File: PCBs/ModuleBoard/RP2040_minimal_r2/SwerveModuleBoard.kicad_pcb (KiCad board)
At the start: 2 copper layers, 60 x 52.9 mm, 57 parts, among them IC1 AS5600-ASOT, J1 USB_B_Micro, J2 Conn_02x02_Counter_Clockwise, J3 Conn_02x08_Odd_Even_MountingP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, J4 Conn_01x07, J5 Conn_01x06_Pin, J6 Conn_01x02, J7 Conn_01x06_Pin, U2 W25Q128JVS, U3 RP2040, U4 DRV8245HQRXZRQ1, U5 DRV8245HQRXZRQ1, U6 MIC5219-3.3YM5, Y1 ABM8-272-T3

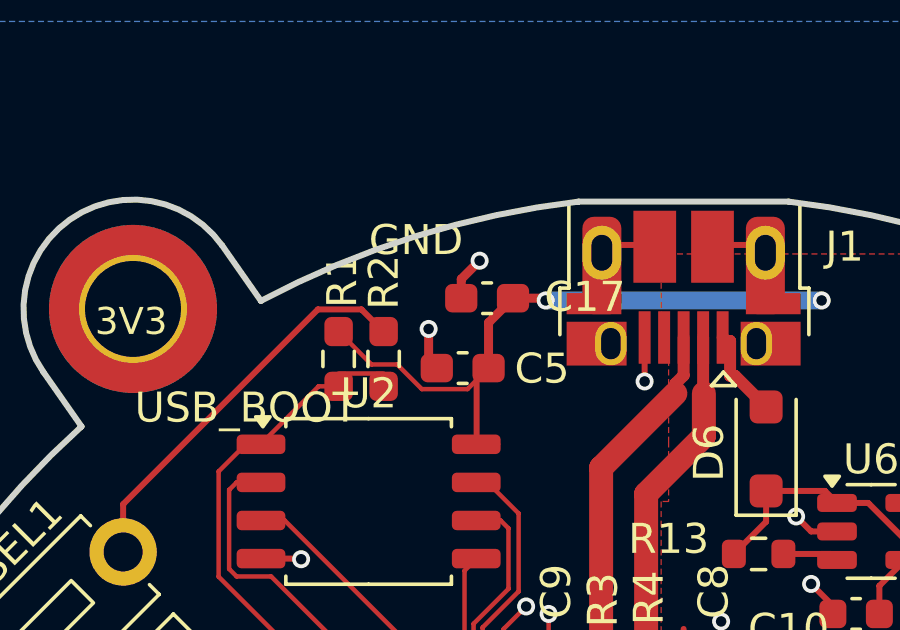
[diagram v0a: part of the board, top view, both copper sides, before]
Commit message: vault backup: 2025-04-25 05:19:58
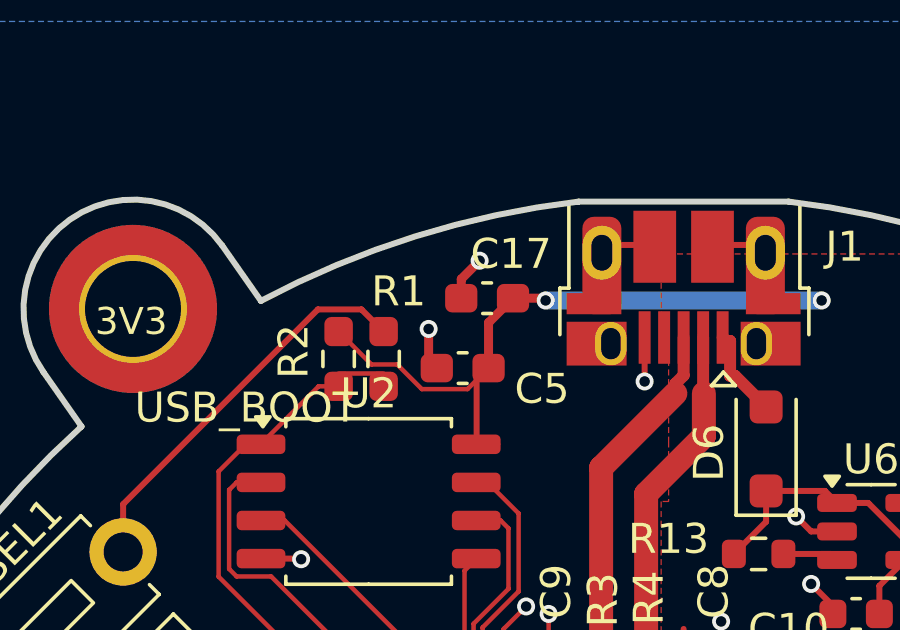
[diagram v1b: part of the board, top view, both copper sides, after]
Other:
- board text removed: "GND"
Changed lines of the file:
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@@
 		(tags "capacitor handsolder")
 		(property "Reference" "C5"
-			(at -2.645 -0.02 180)
+			(at -2.645 -0.695 0)
 			(layer "F.SilkS")
 			(effects
@@
 		(tags "resistor handsolder")
 		(property "Reference" "R2"
-			(at -2.555 -1.51 270)
+			(at -0.25 1.5 270)
 			(layer "F.SilkS")
 			(effects
@@
 		(tags "resistor handsolder")
 		(property "Reference" "R1"
-			(at 2.615 -1.38 90)
+			(at 2.25 0.5 180)
 			(layer "F.SilkS")
 			(effects
@@
 		(tags "capacitor handsolder")
 		(property "Reference" "C17"
-			(at -3.26 0.04 0)
+			(at -0.8 1.475 0)
 			(layer "F.SilkS")
 			(effects
@@
 		)
 	)
-	(gr_text "GND"
-		(at 91.08 71.29 0)
-		(layer "F.SilkS")
-		(effects
-			(font
-				(size 1 1)
-				(thickness 0.15)
-			)
-		)
-	)
 	(gr_text "3V3"
 		(at 81.585 74 0)
@@
 		(min_thickness 0.15)
 		(filled_areas_thickness no)
-		(fill yes
+		(fill
 			(thermal_gap 0.508)
 			(thermal_bridge_width 0.508)
@@
 		(min_thickness 0.15)
 		(filled_areas_thickness no)
-		(fill yes
+		(fill
 			(thermal_gap 0.508)
 			(thermal_bridge_width 0.508)
@@
 		(min_thickness 0.25)
 		(filled_areas_thickness no)
-		(fill yes
+		(fill
 			(thermal_gap 0.5)
 			(thermal_bridge_width 0.5)
@@
 		(min_thickness 0.25)
 		(filled_areas_thickness no)
-		(fill yes
+		(fill
 			(thermal_gap 0.5)
 			(thermal_bridge_width 0.5)
@@
 		(min_thickness 0.2)
 		(filled_areas_thickness no)
-		(fill yes
+		(fill
 			(thermal_gap 0.3)
 			(thermal_bridge_width 0.3)
@@
 		(min_thickness 0.25)
 		(filled_areas_thickness no)
-		(fill yes
+		(fill
 			(thermal_gap 0.5)
 			(thermal_bridge_width 0.5)
